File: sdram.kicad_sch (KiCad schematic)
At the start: 20 parts, among them U1 MT48LC16M16A2P, U8 T8Q144xx

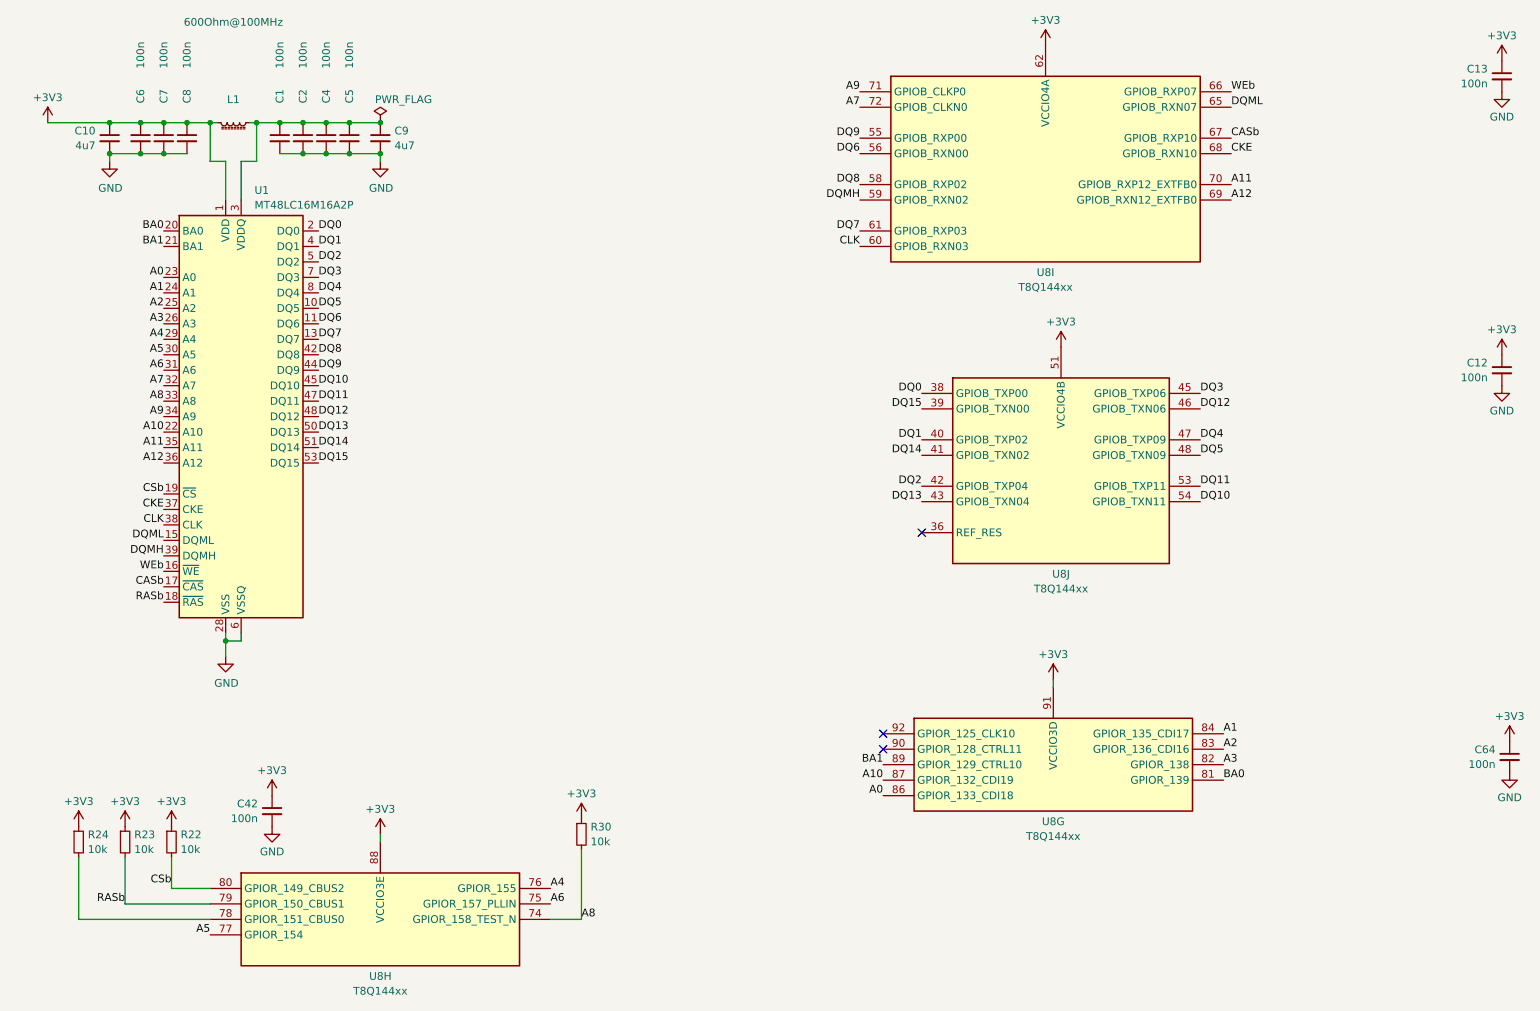
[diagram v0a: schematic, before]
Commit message: layout finished; passed all checks...
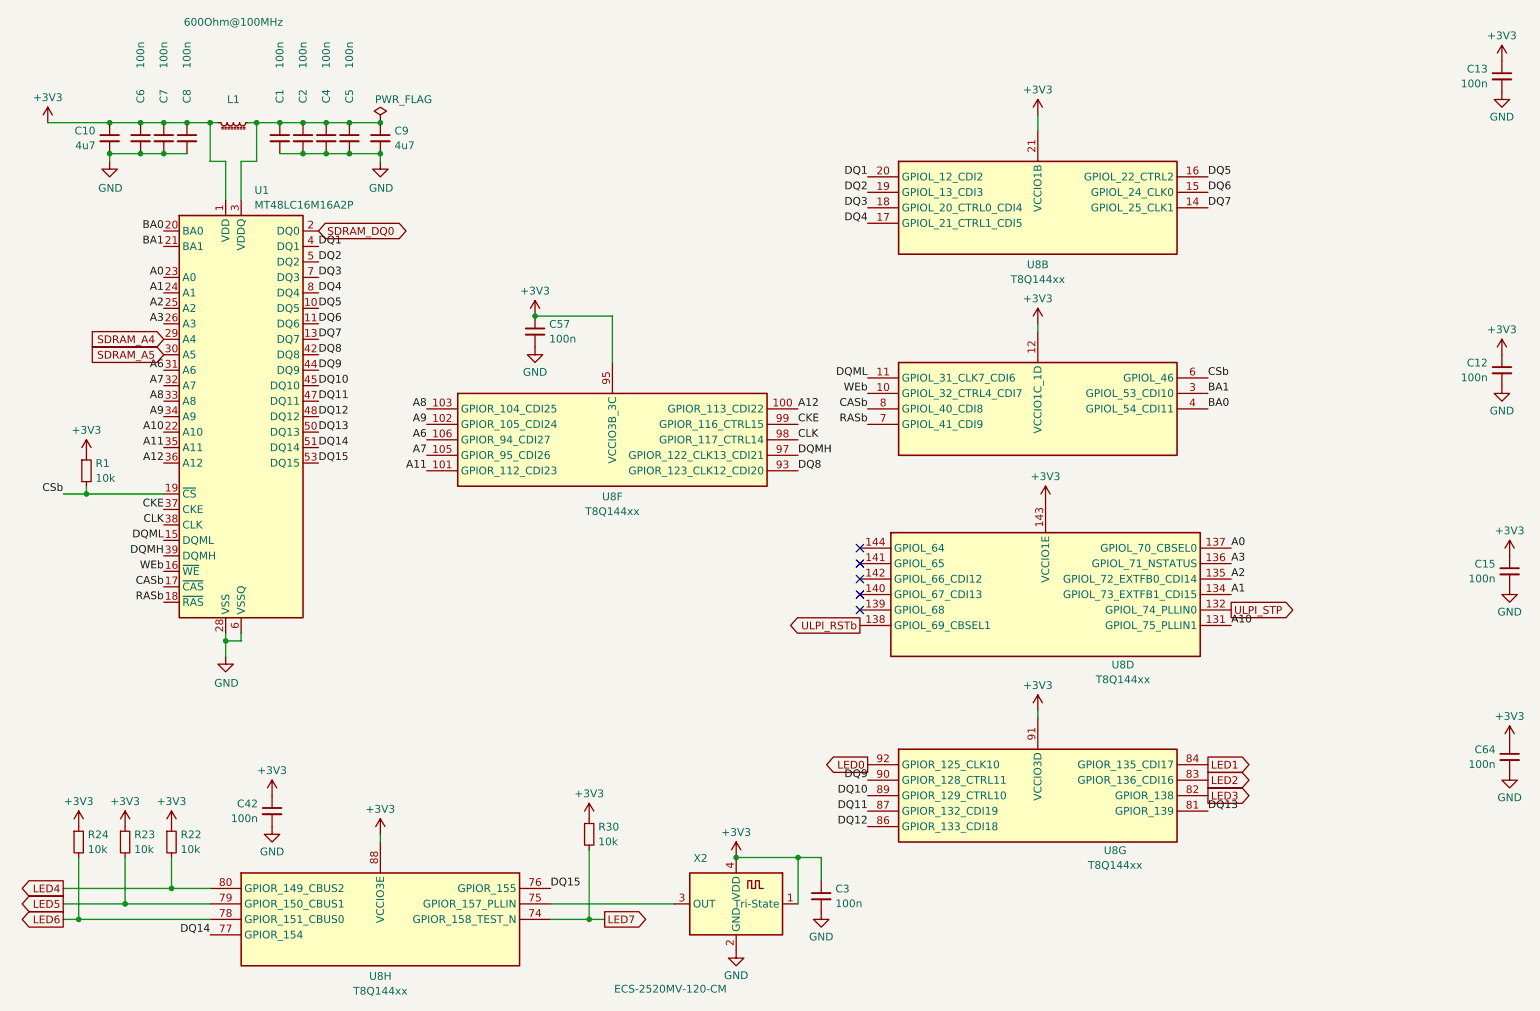
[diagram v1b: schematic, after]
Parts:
- removed unit 10 of U8
- removed unit 9 of U8
- added C15, C3, C57: 100n, Capacitor_SMD:C_0603_1608Metric, symbol Device:C_Small
- added R1: 10k, Resistor_SMD:R_0603_1608Metric, symbol Device:R_Small
- added unit 6 of U8
- added unit 3 of U8
- added unit 4 of U8
- added unit 2 of U8
- added X2: ECS-2520MV-120-CM, Oscillator:Oscillator_SMD_ECS_2520MV-xxx-xx-4Pin_2.5x2.0mm, symbol Oscillator:ECS-2520MV-xxx-xx
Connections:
- net +3V3: now also C15.1, C3.1, C57.1, R1.1, U8.12 (VCCIO1C_1D), U8.143 (VCCIO1E), U8.21 (VCCIO1B), U8.95 (VCCIO3B_3C), X2.1 (Tri-State), X2.4 (VDD)
- net A0: now also U8.137 (GPIOL_70_CBSEL0); no longer U8.86 (GPIOR_133_CDI18)
- net A1: now also U8.134 (GPIOL_73_EXTFB1_CDI15); no longer U8.84 (GPIOR_135_CDI17)
- net A10: now also U8.131 (GPIOL_75_PLLIN1); no longer U8.87 (GPIOR_132_CDI19)
- net A11: now also U8.101 (GPIOR_112_CDI23)
- net A12: now also U8.100 (GPIOR_113_CDI22)
- net A2: now also U8.135 (GPIOL_72_EXTFB0_CDI14); no longer U8.83 (GPIOR_136_CDI16)
- net A3: now also U8.136 (GPIOL_71_NSTATUS); no longer U8.82 (GPIOR_138)
- net A6: now also U8.106 (GPIOR_94_CDI27); no longer U8.75 (GPIOR_157_PLLIN)
- net A7: now also U8.105 (GPIOR_95_CDI26)
- net A8: now also U8.103 (GPIOR_104_CDI25); no longer R30.2, U8.74 (GPIOR_158_TEST_N)
- net A9: now also U8.102 (GPIOR_105_CDI24)
- net BA0: now also U8.4 (GPIOL_54_CDI11); no longer U8.81 (GPIOR_139)
- net BA1: now also U8.3 (GPIOL_53_CDI10); no longer U8.89 (GPIOR_129_CTRL10)
- net CASb: now also U8.8 (GPIOL_40_CDI8)
- net CKE: now also U8.99 (GPIOR_116_CTRL15)
- net CLK: now also U8.98 (GPIOR_117_CTRL14)
- net CSb: now also R1.2, U8.6 (GPIOL_46); no longer R22.2, U8.80 (GPIOR_149_CBUS2)
- net DQ1: now also U8.20 (GPIOL_12_CDI2)
- net DQ10: now also U8.89 (GPIOR_129_CTRL10)
- net DQ11: now also U8.87 (GPIOR_132_CDI19)
- net DQ12: now also U8.86 (GPIOR_133_CDI18)
- net DQ13: now also U8.81 (GPIOR_139)
- net DQ14: now also U8.77 (GPIOR_154)
- net DQ15: now also U8.76 (GPIOR_155)
- net DQ2: now also U8.19 (GPIOL_13_CDI3)
- net DQ3: now also U8.18 (GPIOL_20_CTRL0_CDI4)
- net DQ4: now also U8.17 (GPIOL_21_CTRL1_CDI5)
- net DQ5: now also U8.16 (GPIOL_22_CTRL2)
- net DQ6: now also U8.15 (GPIOL_24_CLK0)
- net DQ7: now also U8.14 (GPIOL_25_CLK1)
- net DQ8: now also U8.93 (GPIOR_123_CLK12_CDI20)
- net DQ9: now also U8.90 (GPIOR_128_CTRL11)
- net DQMH: now also U8.97 (GPIOR_122_CLK13_CDI21)
- net DQML: now also U8.11 (GPIOL_31_CLK7_CDI6)
- net GND: now also C15.2, C3.2, C57.2, X2.2 (GND)
- net RASb: now also U8.7 (GPIOL_41_CDI9); no longer R23.2, U8.79 (GPIOR_150_CBUS1)
- net WEb: now also U8.10 (GPIOL_32_CTRL4_CDI7)
- net LED6: now reaches R24.2, U8.78 (GPIOR_151_CBUS0)
- net LED0: now reaches U8.92 (GPIOR_125_CLK10)
- net A4 renamed SDRAM_A4
- net SDRAM_A4: no longer U8.76 (GPIOR_155)
- net A5 renamed SDRAM_A5
- net SDRAM_A5: no longer U8.77 (GPIOR_154)
- net DQ0 renamed SDRAM_DQ0
- new net: U8.75 (GPIOR_157_PLLIN), X2.3 (OUT)
- new net LED1: U8.84 (GPIOR_135_CDI17)
- new net LED2: U8.83 (GPIOR_136_CDI16)
- new net LED3: U8.82 (GPIOR_138)
- new net LED4: R22.2, U8.80 (GPIOR_149_CBUS2)
- new net LED5: R23.2, U8.79 (GPIOR_150_CBUS1)
- new net LED7: R30.2, U8.74 (GPIOR_158_TEST_N)
- new net ULPI_RSTb: U8.138 (GPIOL_69_CBSEL1)
- new net ULPI_STP: U8.132 (GPIOL_74_PLLIN0)
- no-connect marks 3 -> 5
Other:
- moved on the sheet: R30, U8G
